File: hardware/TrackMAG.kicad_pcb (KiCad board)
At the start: 4 copper layers, 36 x 36 mm, 57 parts, among them J1 USB_C_Socket_USB2.0, J2 Conn_Debug, SW1 SW_RESET, SW2 SW_BOOT, SW3 SW_CALIBRATE, U1 LSM6DS3TR-C, U2 USBLC6-2P6, U3 STM32F103C8T6, U4 LIS2MDL, U5 AMS1117-3.3, Y1 16MHz

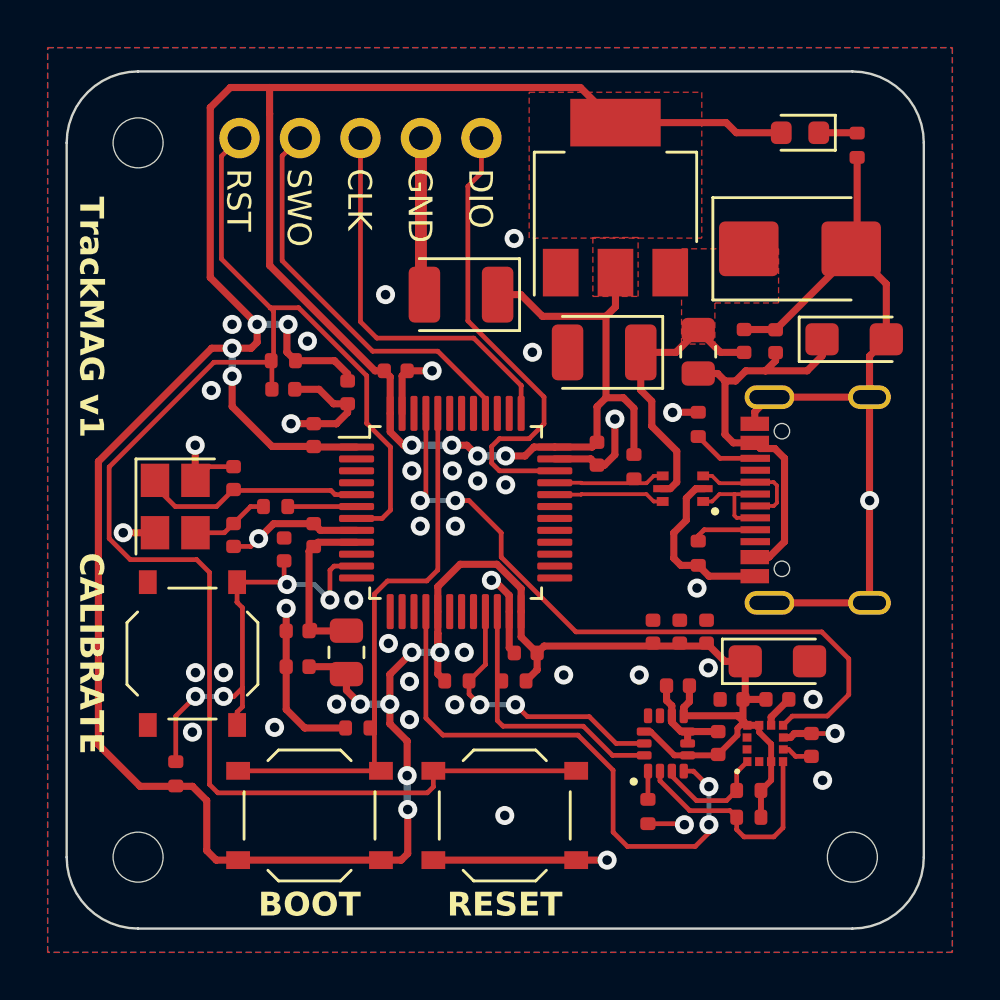
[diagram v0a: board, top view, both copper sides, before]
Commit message: Optimize PCB layout
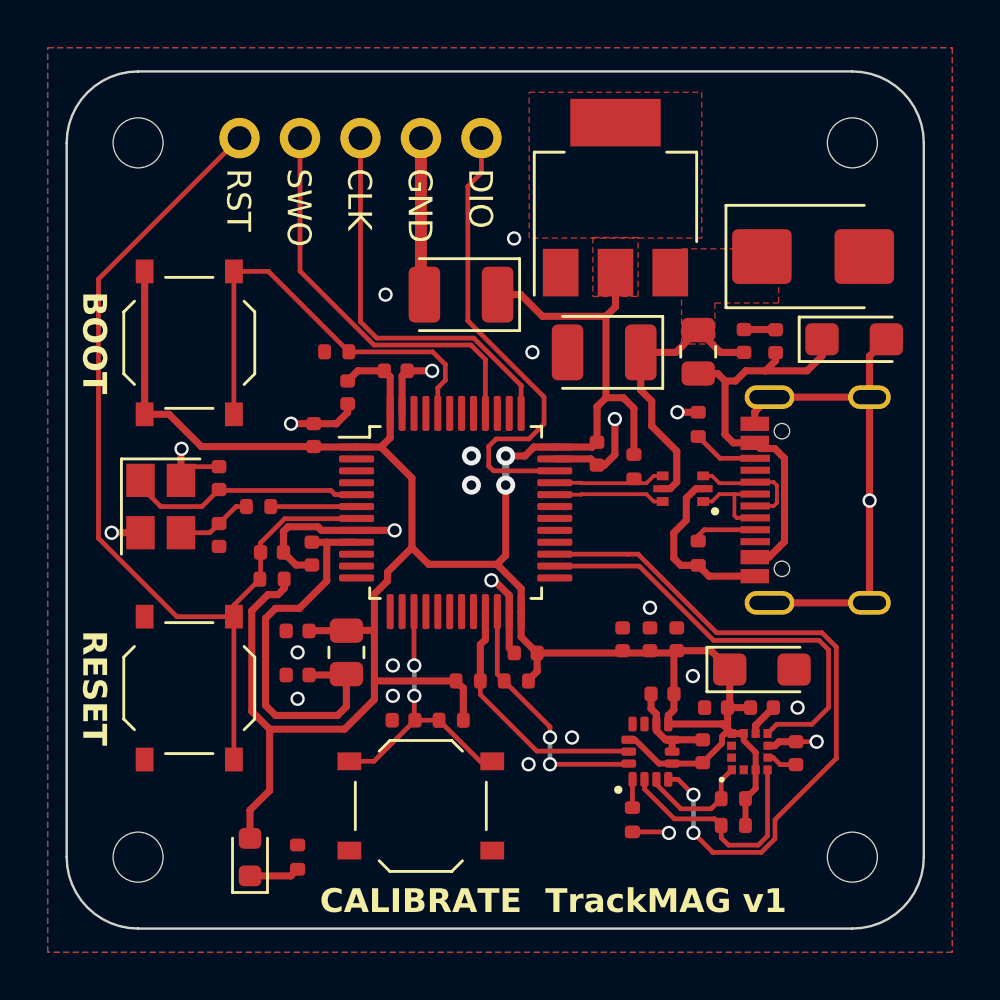
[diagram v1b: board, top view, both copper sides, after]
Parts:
- added H4: MountingHole, MountingHole:MountingHole_2.1mm, F.Cu at (153.8, 74.0)
- moved D1 38.2 mm to (128.5, 104.0), turned to 90 degrees
- moved R13 38.0 mm to (130.5, 104.0), turned to 90 degrees
- moved SW2 20.5 mm to (126.0, 82.4), turned to 90 degrees
- moved R7 15.8 mm to (132.1, 82.8)
- moved SW1 14.3 mm to (126.0, 96.9), turned to 90 degrees
- moved R12 11.8 mm to (136.9, 98.2), turned to 0 degrees
- moved SW3 11.5 mm to (135.7, 101.8), turned to 180 degrees
- moved R1 9.19 mm to (129.4, 92.3)
- moved C23 8.76 mm to (134.9, 98.2), turned to 180 degrees
- moved C17 6.87 mm to (129.4, 91.2)
- moved C15 1.85 mm to (130.5, 96.3)
- moved C16 1.50 mm to (130.5, 94.5)
- moved C3 1.31 mm to (144.2, 94.8)
- moved C1 1.29 mm to (146.4, 94.8)
- moved C2 1.29 mm to (145.3, 94.8)
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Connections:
- U3 pad 11: CALIBRATE -> unconnected-(U3-PA1-Pad11)
- U3 pad 15: unconnected-(U3-PA5-Pad15) -> CALIBRATE
- U3 pad 16: INT1 -> unconnected-(U3-PA6-Pad16)
- U3 pad 17: +3.3V -> unconnected-(U3-PA7-Pad17)
- U3 pad 26: unconnected-(U3-PB13-Pad26) -> DRDY
- U3 pad 27: unconnected-(U3-PB14-Pad27) -> INT1
- U3 pad 45: DRDY -> unconnected-(U3-PB8-Pad45)
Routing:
- net +3.3V: track 185.5 -> 121.9 mm, vias 14 -> 2
- net GND: track 101.8 -> 72.8 mm, vias 43 -> 25
- net RESET: track 66.4 -> 40.3 mm
- net DRDY: track 30.1 -> 18.4 mm, vias 2 -> 0
- net +3.3VA: track 7.35 -> 16.9 mm
- net CALIBRATE: track 19.1 -> 12.0 mm, vias 4 -> 2
- net INT1: track 23.6 -> 29.5 mm
- net /BOOT0: track 24.5 -> 18.7 mm
- net I2C2_SCL: track 12.1 -> 10.8 mm, vias 2 -> 0
- net I2C2_SDA: track 11.3 -> 10.7 mm, vias 0 -> 2
- net /HSE_IN: track 9.55 -> 10.2 mm
- net /HSE_O: track 2.89 -> 3.43 mm
